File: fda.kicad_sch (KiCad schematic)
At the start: 43 parts, among them U706 OPA2197D, U73 OPA2388DGK, U74 THS4521IDGK

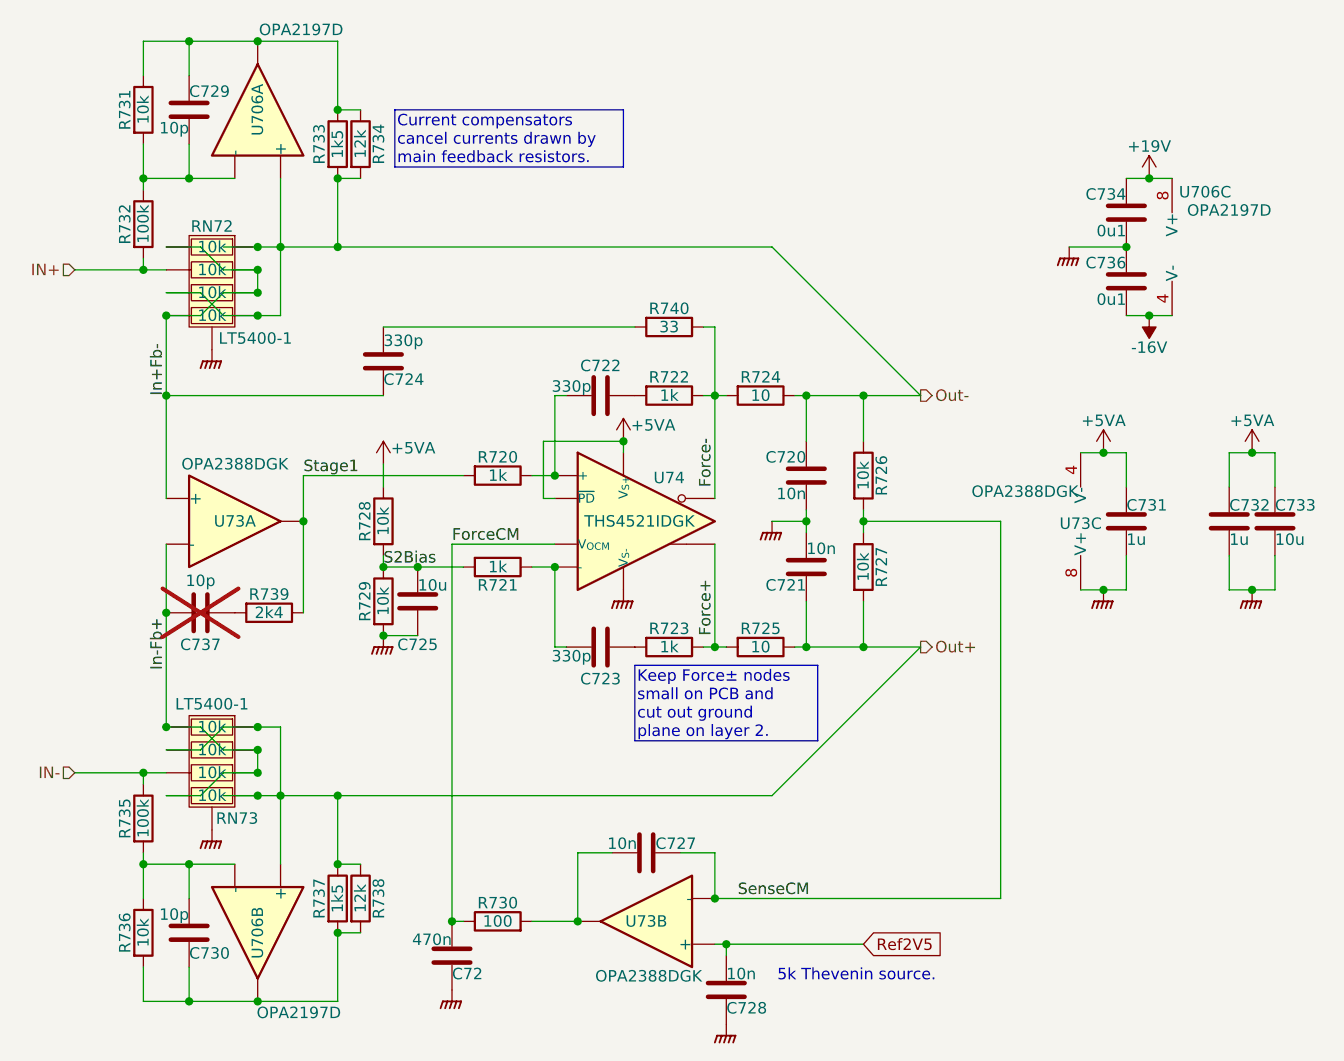
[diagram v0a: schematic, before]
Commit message: Adjust placements
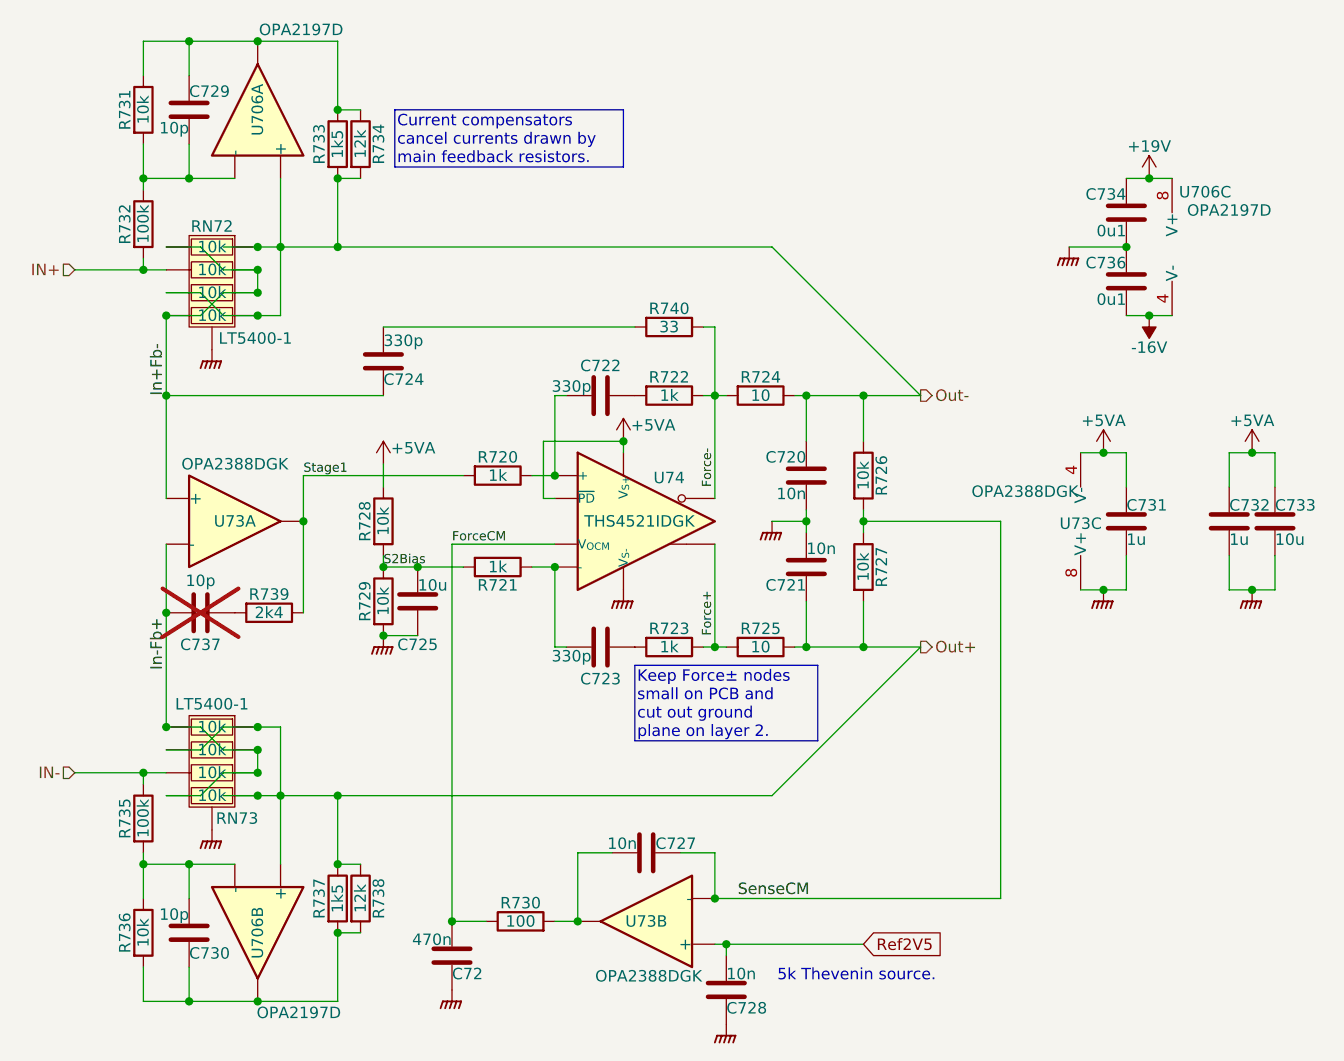
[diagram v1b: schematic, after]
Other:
- moved on the sheet: R730
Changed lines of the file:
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@@
 	(wire
 		(pts
-			(xy 113.03 148.59) (xy 118.11 148.59)
+			(xy 115.57 148.59) (xy 118.11 148.59)
 		)
 		(stroke
@@
 	(wire
 		(pts
-			(xy 104.14 148.59) (xy 105.41 148.59)
+			(xy 104.14 148.59) (xy 107.95 148.59)
 		)
 		(stroke
@@
 		(effects
 			(font
-				(size 1.27 1.27)
+				(size 1.016 1.016)
 			)
 			(justify left bottom)
@@
 		(effects
 			(font
-				(size 1.27 1.27)
+				(size 1.016 1.016)
 			)
 			(justify left bottom)
@@
 		(effects
 			(font
-				(size 1.27 1.27)
+				(size 1.016 1.016)
 			)
 			(justify left bottom)
@@
 		(effects
 			(font
-				(size 1.27 1.27)
+				(size 1.016 1.016)
 			)
 			(justify left bottom)
@@
 		(effects
 			(font
-				(size 1.27 1.27)
+				(size 1.016 1.016)
 			)
 			(justify left bottom)
@@
 	(symbol
 		(lib_id "Device:R")
-		(at 109.22 148.59 90)
+		(at 111.76 148.59 90)
 		(unit 1)
 		(exclude_from_sim no)
@@
 		(dnp no)
 		(property "Reference" "R730"
-			(at 109.22 146.558 90)
+			(at 111.76 146.558 90)
 			(effects
 				(font
@@
 		)
 		(property "Value" "100"
-			(at 109.22 148.59 90)
+			(at 111.76 148.59 90)
 			(effects
 				(font
@@
 		)
 		(property "Footprint" "Resistor_SMD:R_0402_1005Metric"
-			(at 109.22 150.368 90)
+			(at 111.76 150.368 90)
 			(effects
 				(font
@@
 		)
 		(property "Datasheet" "~"
-			(at 109.22 148.59 0)
+			(at 111.76 148.59 0)
 			(effects
 				(font
@@
 		)
 		(property "Description" "Resistor"
-			(at 109.22 148.59 0)
+			(at 111.76 148.59 0)
 			(effects
 				(font
@@
 		)
 		(property "LCSC" "C25076"
-			(at 109.22 148.59 90)
+			(at 111.76 148.59 90)
 			(effects
 				(font
@@
 		)
 		(property "Stock" ""
-			(at 109.22 148.59 90)
+			(at 111.76 148.59 90)
 			(effects
 				(font
